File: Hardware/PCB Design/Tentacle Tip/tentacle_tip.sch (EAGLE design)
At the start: 8 parts, among them U1 ADXL345

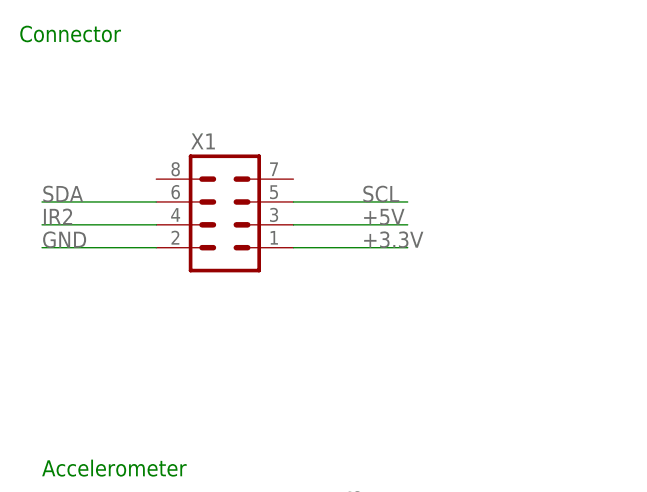
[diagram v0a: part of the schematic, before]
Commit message: Updated the board design
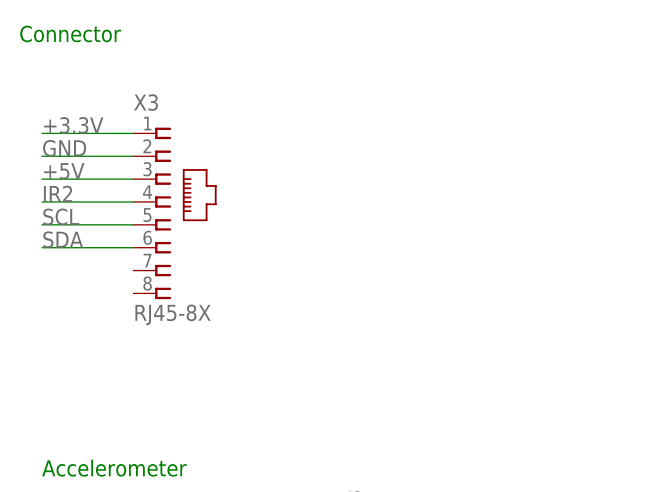
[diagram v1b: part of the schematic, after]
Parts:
- removed X1: (no value), CBLA_Test_bed_Library:MA04-2
- added X3: RJ45-8X, CBLA_Test_bed_Library:RJ45-8X
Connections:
- net +3.3V: now also X3.1; no longer X1.1
- net +5V: now also X3.3; no longer X1.3
- net GND: now also X3.2; no longer X1.2
- net IR2: now also X3.4; no longer X1.4
- net SCL: now also X3.5; no longer X1.5
- net SDA: now also X3.6; no longer X1.6
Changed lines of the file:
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@@
 <part name="X2" library="CBLA_Test_bed_Library" deviceset="PINHD-1X3" device="/90"/>
 <part name="GND5" library="supply1" deviceset="GND" device=""/>
-<part name="X1" library="CBLA_Test_bed_Library" deviceset="MA04-2" device=""/>
+<part name="X3" library="CBLA_Test_bed_Library" deviceset="RJ45" device="" technology="-8X"/>
 </parts>
 <sheets>
@@
 <instance part="X2" gate="A" x="187.96" y="93.98" rot="R180"/>
 <instance part="GND5" gate="1" x="165.1" y="83.82"/>
-<instance part="X1" gate="G$1" x="50.8" y="147.32"/>
+<instance part="X3" gate="G$1" x="43.18" y="147.32"/>
 </instances>
 <busses>
@@
 </segment>
 <segment>
-<pinref part="X1" gate="G$1" pin="4"/>
-<wire x1="43.18" y1="144.78" x2="30.48" y2="144.78" width="0.1524" layer="91"/>
-<label x="30.48" y="144.78" size="1.778" layer="95"/>
+<pinref part="X3" gate="G$1" pin="4"/>
+<wire x1="40.64" y1="147.32" x2="30.48" y2="147.32" width="0.1524" layer="91"/>
+<label x="30.48" y="147.32" size="1.778" layer="95"/>
 </segment>
 </net>
@@
 </segment>
 <segment>
-<pinref part="X1" gate="G$1" pin="3"/>
-<wire x1="58.42" y1="144.78" x2="71.12" y2="144.78" width="0.1524" layer="91"/>
-<label x="66.04" y="144.78" size="1.778" layer="95"/>
+<pinref part="X3" gate="G$1" pin="3"/>
+<wire x1="40.64" y1="149.86" x2="30.48" y2="149.86" width="0.1524" layer="91"/>
+<label x="30.48" y="149.86" size="1.778" layer="95"/>
 </segment>
 </net>
@@
 </segment>
 <segment>
-<pinref part="X1" gate="G$1" pin="1"/>
-<wire x1="58.42" y1="142.24" x2="71.12" y2="142.24" width="0.1524" layer="91"/>
-<label x="66.04" y="142.24" size="1.778" layer="95"/>
-</segment>
-<segment>
 <pinref part="+3V34" gate="G$1" pin="+3V3"/>
 <wire x1="104.14" y1="111.76" x2="104.14" y2="106.68" width="0.1524" layer="91"/>
@@
 <wire x1="111.76" y1="106.68" x2="119.38" y2="106.68" width="0.1524" layer="91"/>
 <junction x="111.76" y="106.68"/>
+</segment>
+<segment>
+<pinref part="X3" gate="G$1" pin="1"/>
+<wire x1="40.64" y1="154.94" x2="30.48" y2="154.94" width="0.1524" layer="91"/>
+<label x="30.48" y="154.94" size="1.778" layer="95"/>
 </segment>
 </net>
@@
 </segment>
 <segment>
-<pinref part="X1" gate="G$1" pin="2"/>
-<wire x1="43.18" y1="142.24" x2="30.48" y2="142.24" width="0.1524" layer="91"/>
-<label x="30.48" y="142.24" size="1.778" layer="95"/>
+<pinref part="X3" gate="G$1" pin="2"/>
+<wire x1="40.64" y1="152.4" x2="30.48" y2="152.4" width="0.1524" layer="91"/>
+<label x="30.48" y="152.4" size="1.778" layer="95"/>
 </segment>
 </net>
@@
 </segment>
 <segment>
-<pinref part="X1" gate="G$1" pin="5"/>
-<wire x1="58.42" y1="147.32" x2="71.12" y2="147.32" width="0.1524" layer="91"/>
-<label x="66.04" y="147.32" size="1.778" layer="95"/>
+<pinref part="X3" gate="G$1" pin="5"/>
+<wire x1="40.64" y1="144.78" x2="30.48" y2="144.78" width="0.1524" layer="91"/>
+<label x="30.48" y="144.78" size="1.778" layer="95"/>
 </segment>
 </net>
@@
 </segment>
 <segment>
-<pinref part="X1" gate="G$1" pin="6"/>
-<wire x1="43.18" y1="147.32" x2="30.48" y2="147.32" width="0.1524" layer="91"/>
-<label x="30.48" y="147.32" size="1.778" layer="95"/>
+<pinref part="X3" gate="G$1" pin="6"/>
+<wire x1="40.64" y1="142.24" x2="30.48" y2="142.24" width="0.1524" layer="91"/>
+<label x="30.48" y="142.24" size="1.778" layer="95"/>
 </segment>
 </net>
